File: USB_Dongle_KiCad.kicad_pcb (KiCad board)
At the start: 6 copper layers, 63.6 x 27.1 mm, 56 parts, among them J1 USB_C_Receptacle_USB2.0, J2 Conn SWD 02x05, J3 DM3BT-DSF-PEJS, SW1 PCM12SMTR, SW2 KMR223G LFG, U1 AMS1117-3.3, U2 STULPI01A, U3 USBULC6-2M6, U4 ESDA14V2-2BF3, U5 STM32F730R8Tx, U6 CAT811TTBI-GT3, Y1 3225 SMD Oscillator, Y2 24MHz / 10pF / 20ppm

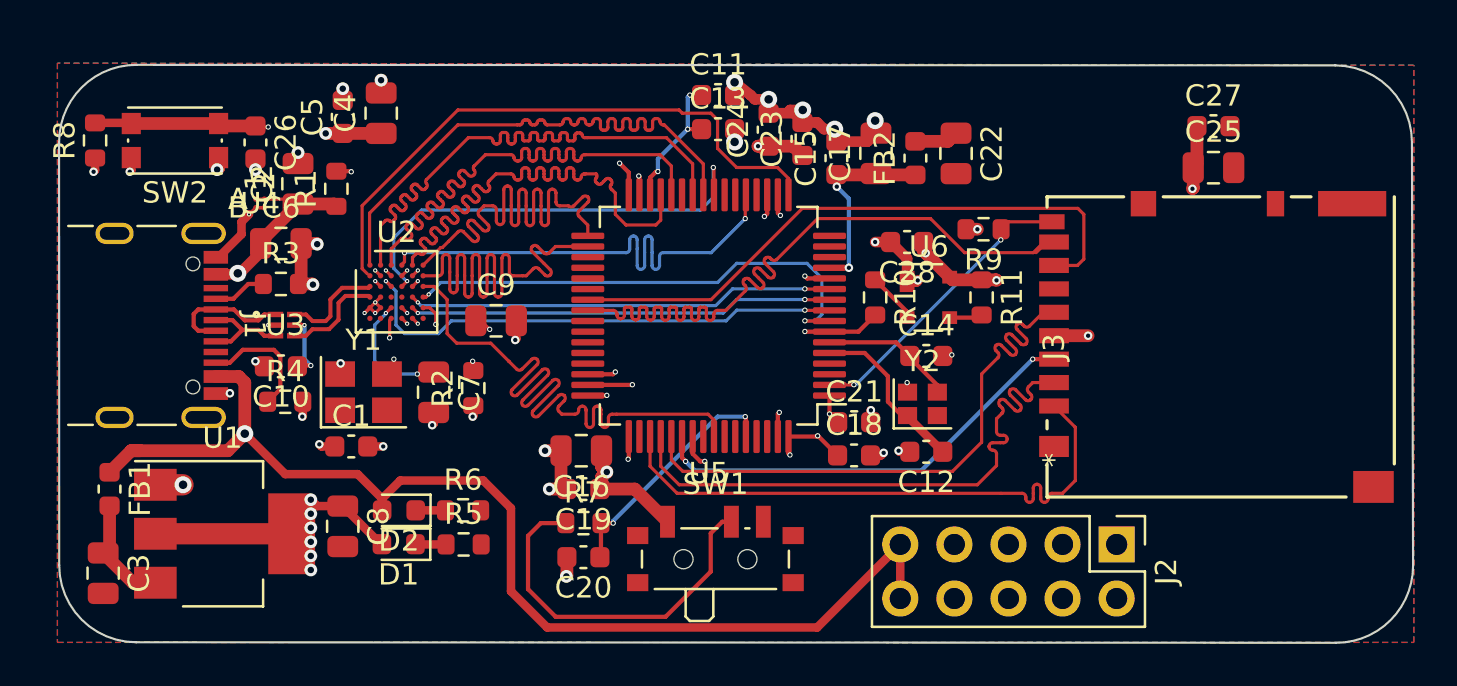
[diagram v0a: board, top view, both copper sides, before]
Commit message: Various fixes and other 3D models added
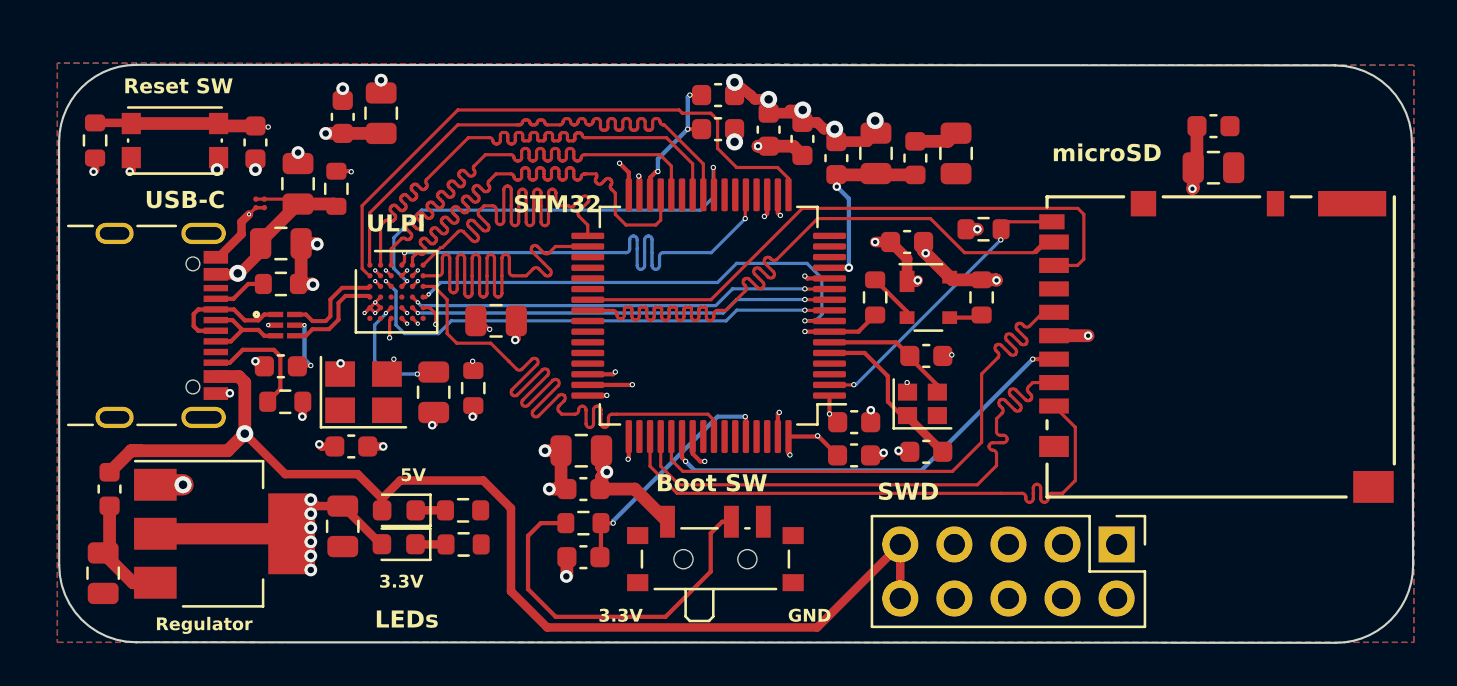
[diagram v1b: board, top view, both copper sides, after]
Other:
- board text added: "3.3V"
- board text added: "5V"
- board text added: "Boot SW"
- board text added: "GND"
- board text added: "LEDs"
- board text added: "Regulator"
- board text added: "Reset SW"
- board text added: "STM32"
- board text added: "SWD"
- board text added: "ULPI"
- board text added: "USB-C"
- board text added: "microSD"
